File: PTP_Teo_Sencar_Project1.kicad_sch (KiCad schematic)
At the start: 45 parts, among them J1 Screw_Terminal_01x02, SW1 SW_Push, SW2 SW_SPDT_312, U1 LM2574N-5, U2 4027, U3 4027, U4 74LS47, U5 FYS-3911BUHR-21, U6 74LVC1G11, U7 NE555P

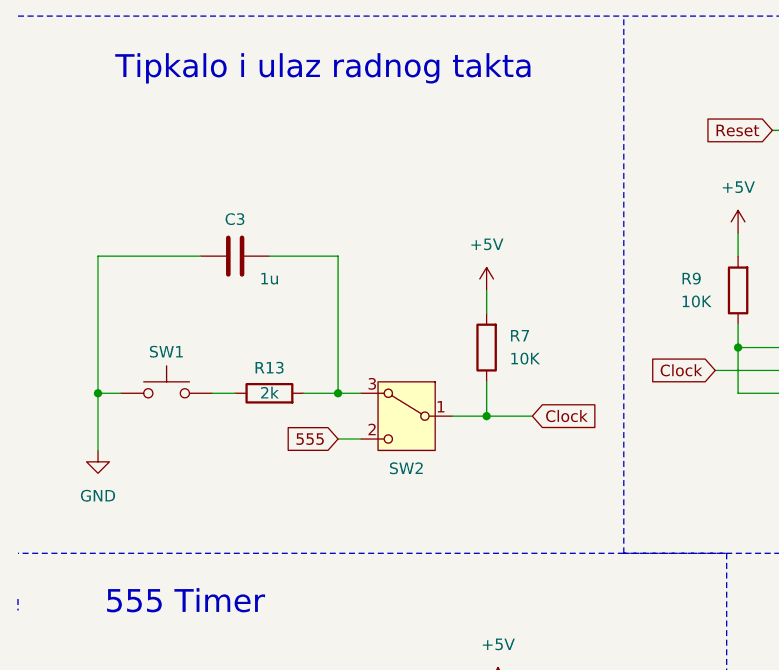
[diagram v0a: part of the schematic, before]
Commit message: Gerber fileovi, BOM
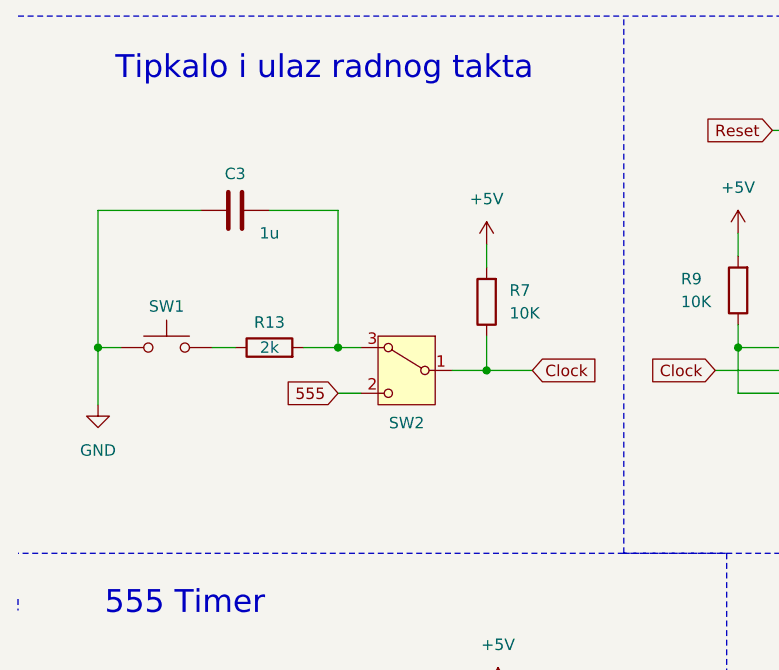
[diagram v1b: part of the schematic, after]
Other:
- moved on the sheet: C3, R13, R7, SW1, SW2
